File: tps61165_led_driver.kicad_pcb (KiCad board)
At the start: 2 copper layers, 12 parts, among them K1 CONN_3, P1 CONN_2, U1 TPS61165_DBV_6_DBV6

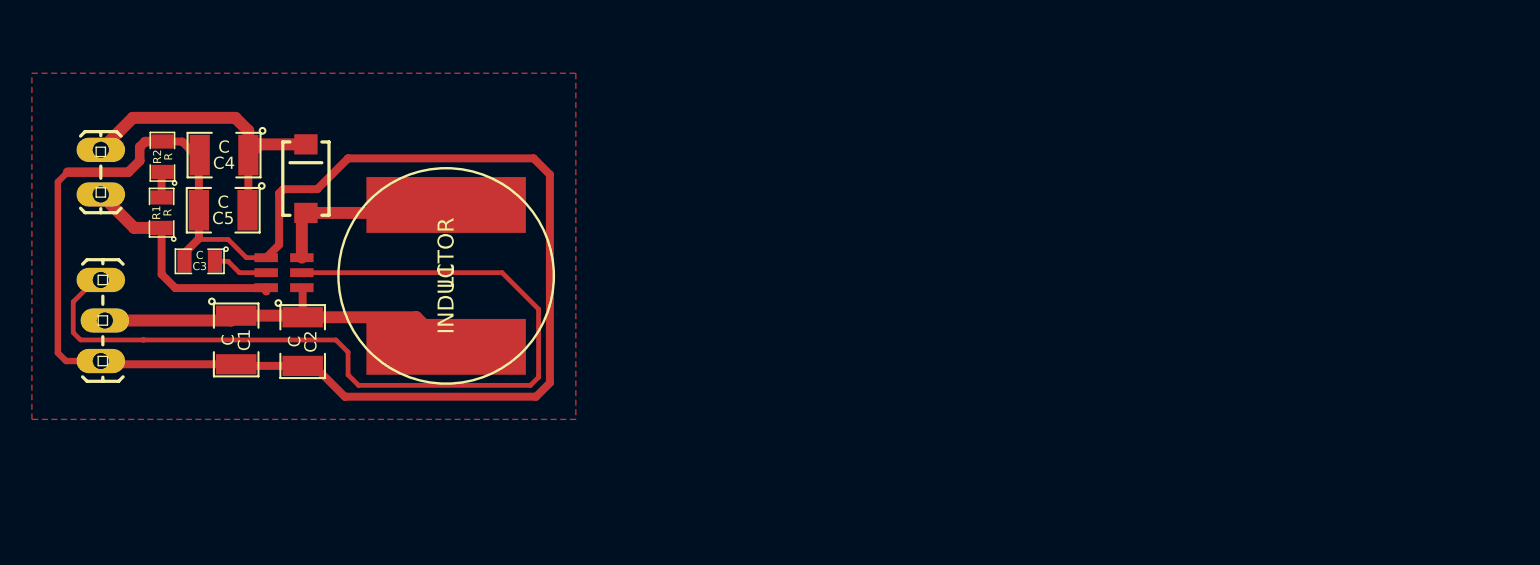
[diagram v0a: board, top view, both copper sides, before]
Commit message: ADD: pdf
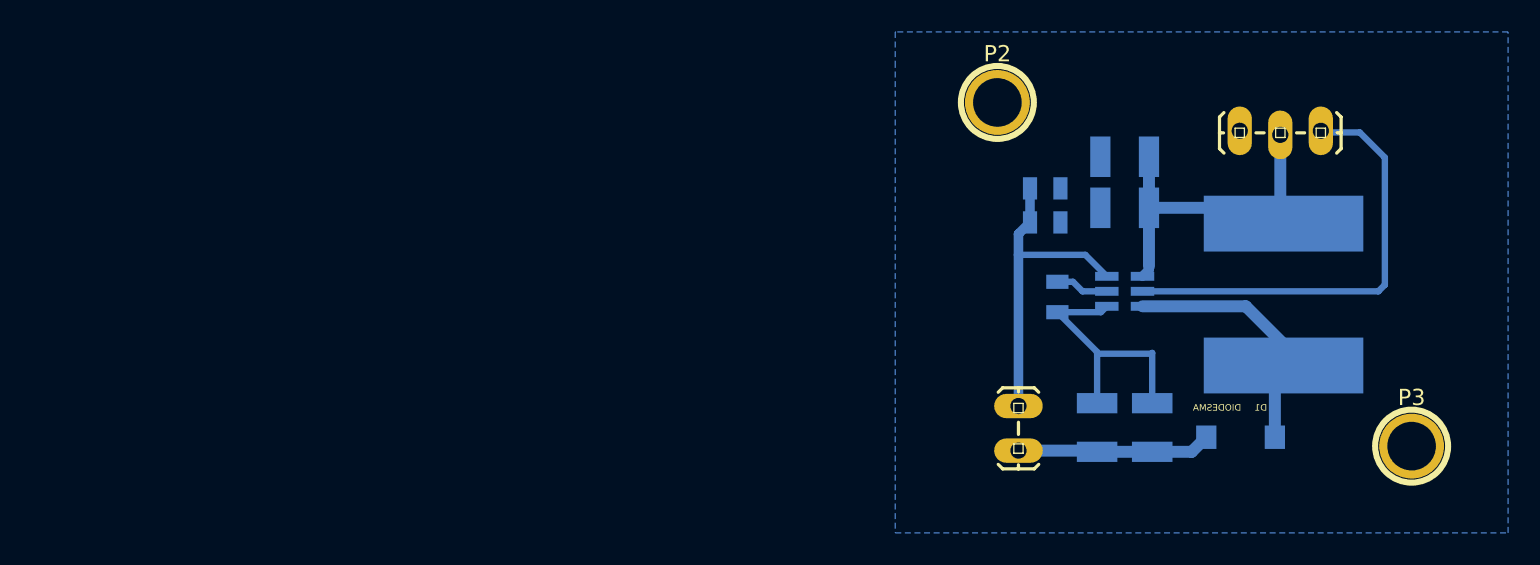
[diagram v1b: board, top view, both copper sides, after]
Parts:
- added P2: CONN_1, 1pin, F.Cu at (172.7, 117.2)
- added P3: CONN_1, 1pin, F.Cu at (198.6, 138.8)
- C1, C2, C3, C4, C5, D1, L1, R1, R2, U1: moved to B.Cu
- moved K1 72.8 mm to (187.9, 119.0), turned to 0 degrees
- moved D1 60.8 mm to (187.9, 138.2), turned to 180 degrees
- moved C4 60.6 mm to (182.4, 137.6), turned to 90 degrees
- moved P1 59.1 mm to (174.0, 136.4), turned to 270 degrees
- moved C5 56.4 mm to (178.9, 137.6), turned to 90 degrees
- moved C1 56.3 mm to (180.6, 123.9), turned to 180 degrees
- moved R2 55.5 mm to (175.7, 124.8), turned to 0 degrees
- moved R1 55.4 mm to (175.7, 122.6), turned to 0 degrees
- moved C3 53.8 mm to (176.4, 129.4), turned to 270 degrees
- moved C2 52.8 mm to (180.6, 120.7), turned to 180 degrees
- moved U1 52.7 mm to (180.6, 129.1)
- moved L1 52.5 mm to (190.6, 129.3), turned to 90 degrees
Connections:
- net N-000007 renamed /Comp
- net N-000008 renamed /Vin
- C1 pad 2: N-000009 -> /GND
- C2 pad 2: N-000009 -> /GND
- C3 pad 2: N-000009 -> /GND
- C4 pad 2: N-000009 -> /GND
- C5 pad 2: N-000009 -> /GND
- K1 pad 1: N-000009 -> /GND
- K1 pad 3: N-000005 (its old number) -> /Ctrl
- P1 pad 1: N-000002 -> /FB
- R1 pad 1: N-000002 -> /FB
- R1 pad 2: N-000001 -> /GND
- R2 pad 1: N-000001 -> /FB
- R2 pad 2: N-000009 -> /GND
- U1 pad 2: N-000005 (its old number) -> /Ctrl
- U1 pad 4: N-000009 -> /GND
- U1 pad 6: N-000002 -> /FB
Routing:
- net N-000009: track 103.1 -> 0.00 mm
- net N-000005 (its old number): track 55.9 -> 0.00 mm
- net /Ctrl: track 0.00 -> 28.0 mm
- net /FB: track 0.00 -> 20.0 mm
- net /GND: track 0.00 -> 16.6 mm
- net N-000002: track 15.0 -> 0.00 mm
- net /Out: track 19.3 -> 12.2 mm
- net N-000005: track 11.9 -> 15.9 mm
- net N-000001: track 1.62 -> 0.00 mm
- net /Vin: track 24.2 -> 23.5 mm
- added copper zone on B.Cu, net /GND
- removed copper zone on F.Cu, net N-000009
